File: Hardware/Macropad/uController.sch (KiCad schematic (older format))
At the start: 16 parts, among them J3 Conn_02x03_Odd_Even, SW22 SW_Push, U5 ATmega32U4-AU, X1 KC2016K

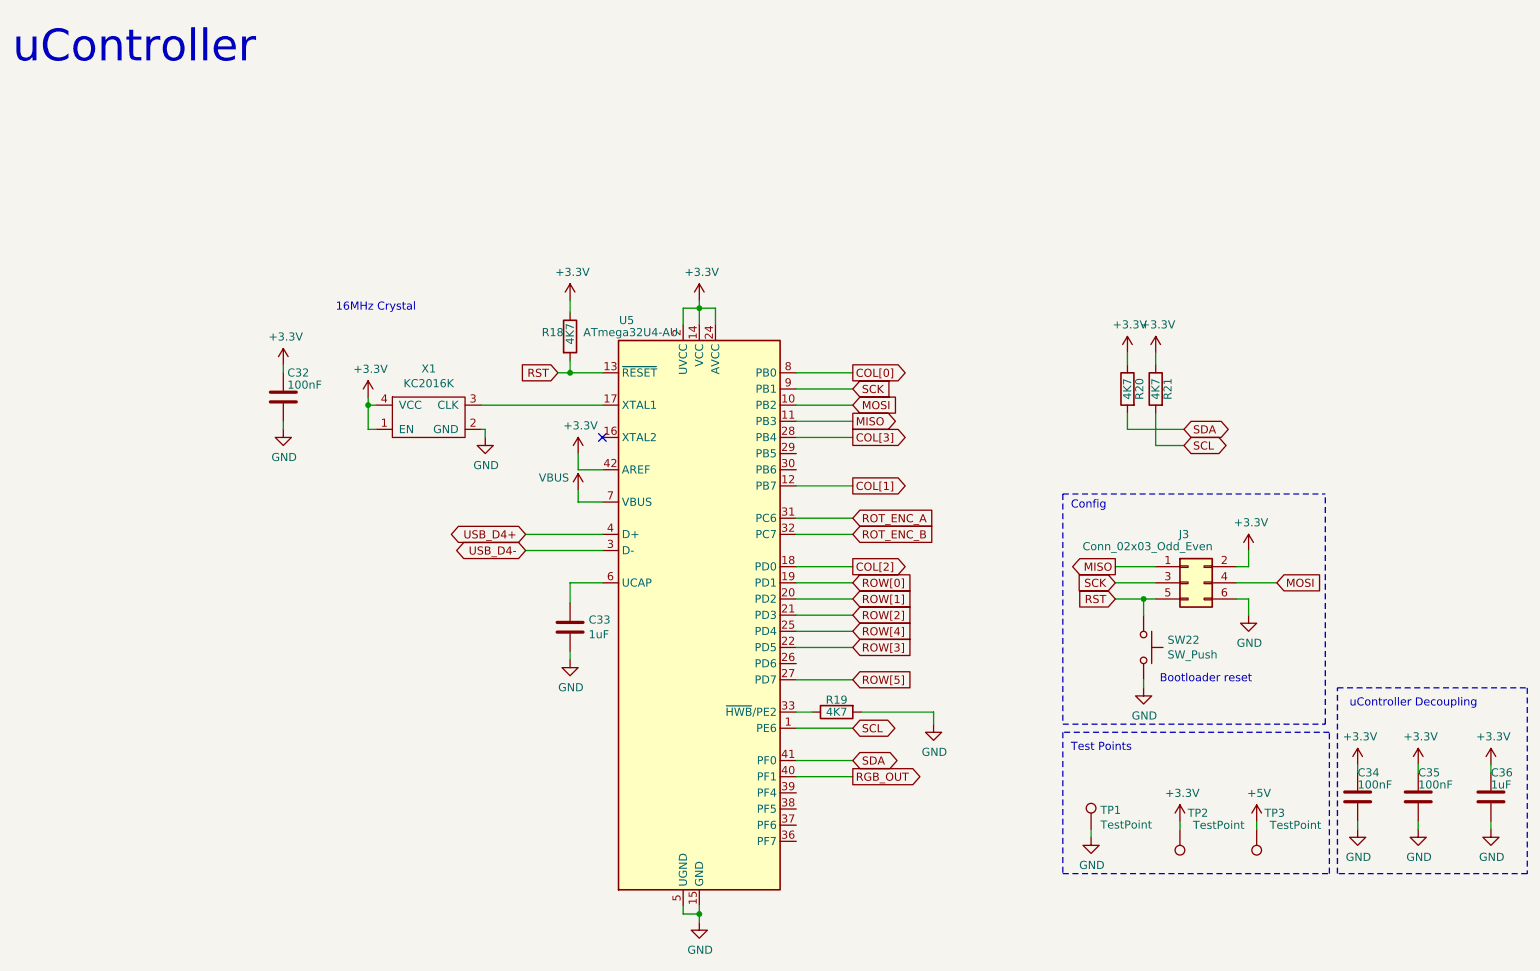
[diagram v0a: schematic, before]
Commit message: Layout done, cleaned up schematic and generated gerbers
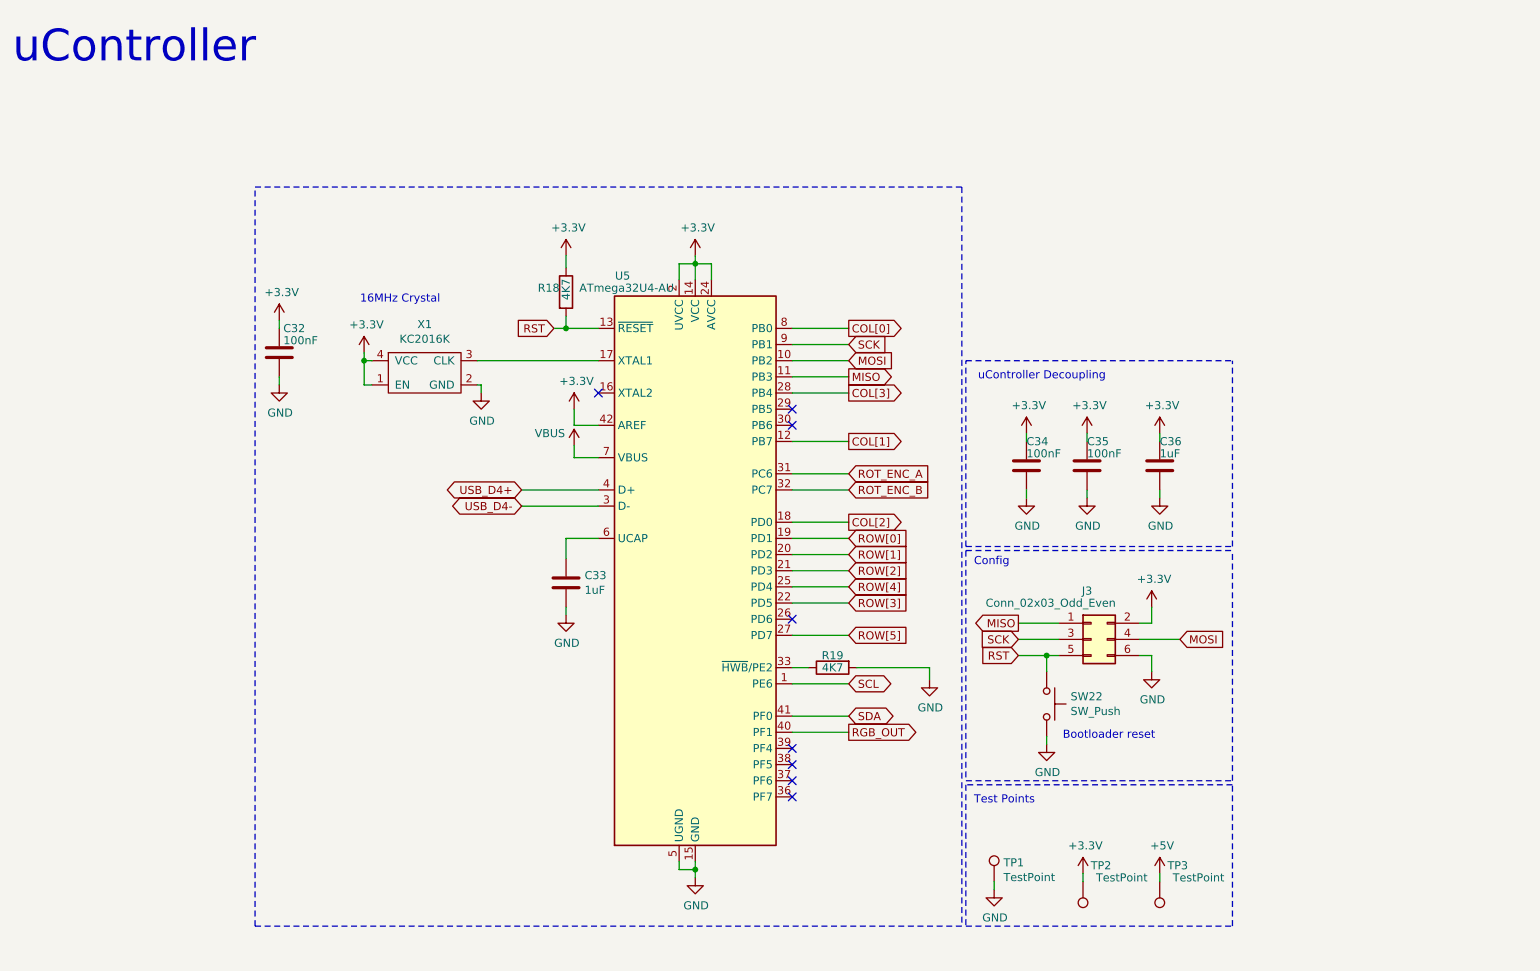
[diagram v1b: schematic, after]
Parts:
- removed R20, R21: 4K7, resistor_smd:R_0603_1608Metric, symbol Device:R
- SW22: footprint button_switch_smd:SW_SPST_B3U-1000P -> custom_footprint_library:SW_SPST_B3U-1000P
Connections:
- no-connect marks 1 -> 8
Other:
- moved on the sheet: C32, C33, C34, C35, C36, J3, R18, R19, SW22, TP1, TP2, TP3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
